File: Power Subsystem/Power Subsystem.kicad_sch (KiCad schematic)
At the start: 38 parts, among them J1 Conn_01x16_Pin, J2 Conn_01x02_Pin, Q1 PMOS, SW1 SW_SPST, U1 MCP73831-2-OT

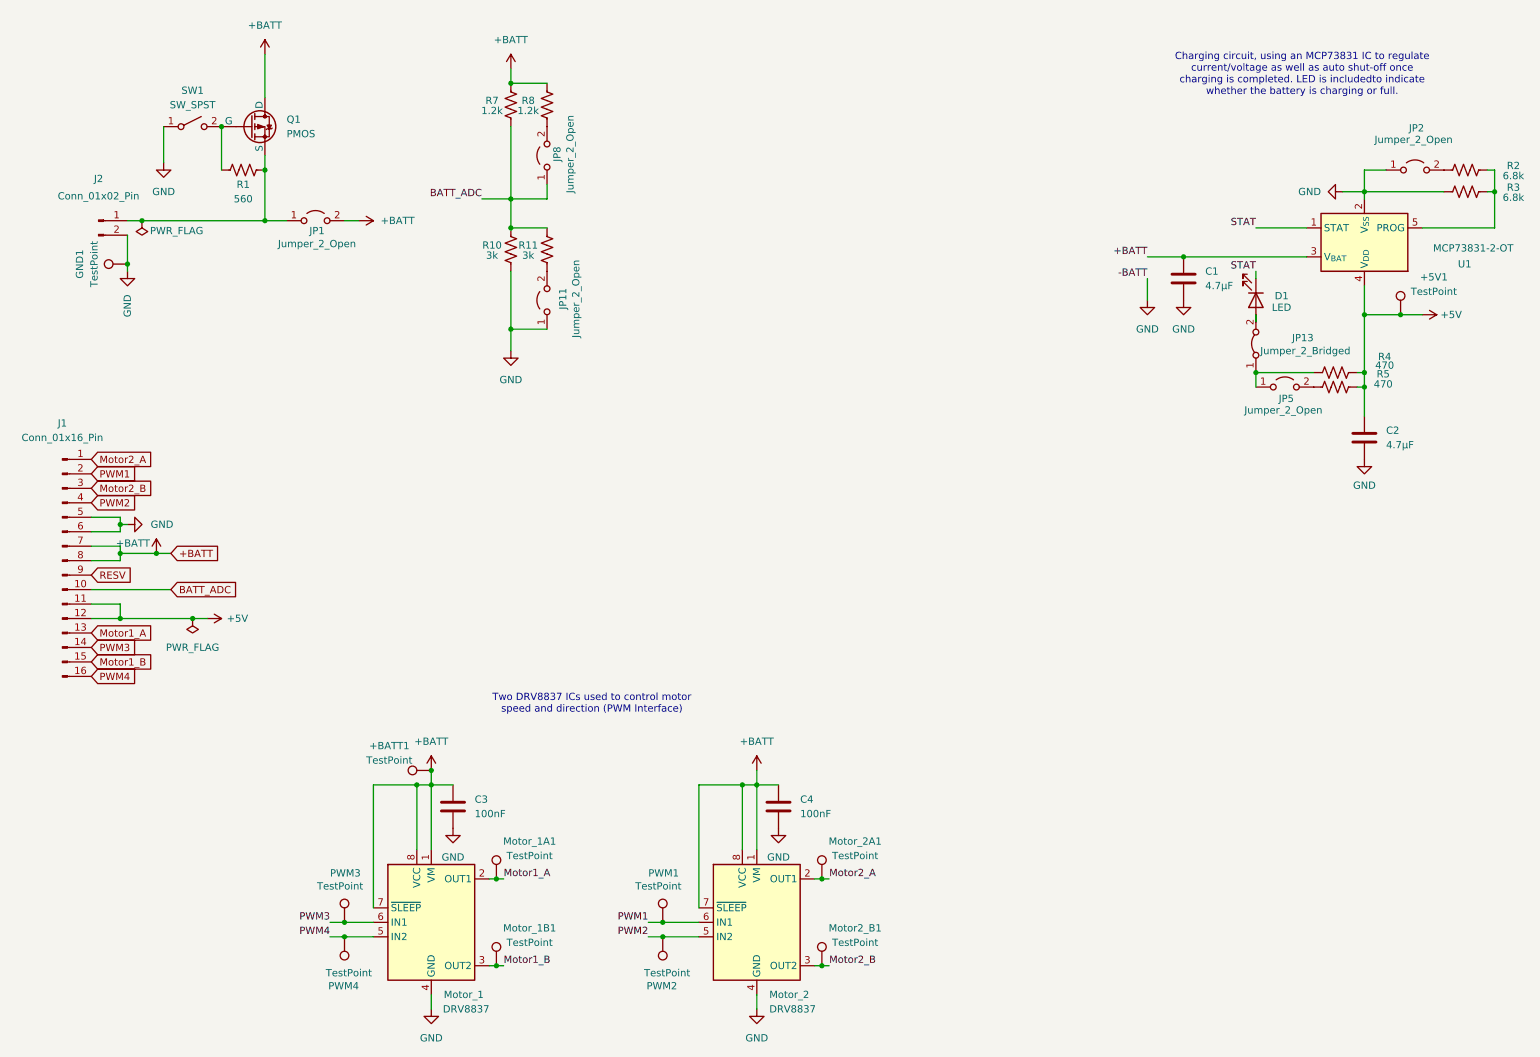
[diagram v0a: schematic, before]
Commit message: Final Schematic and PCB designs
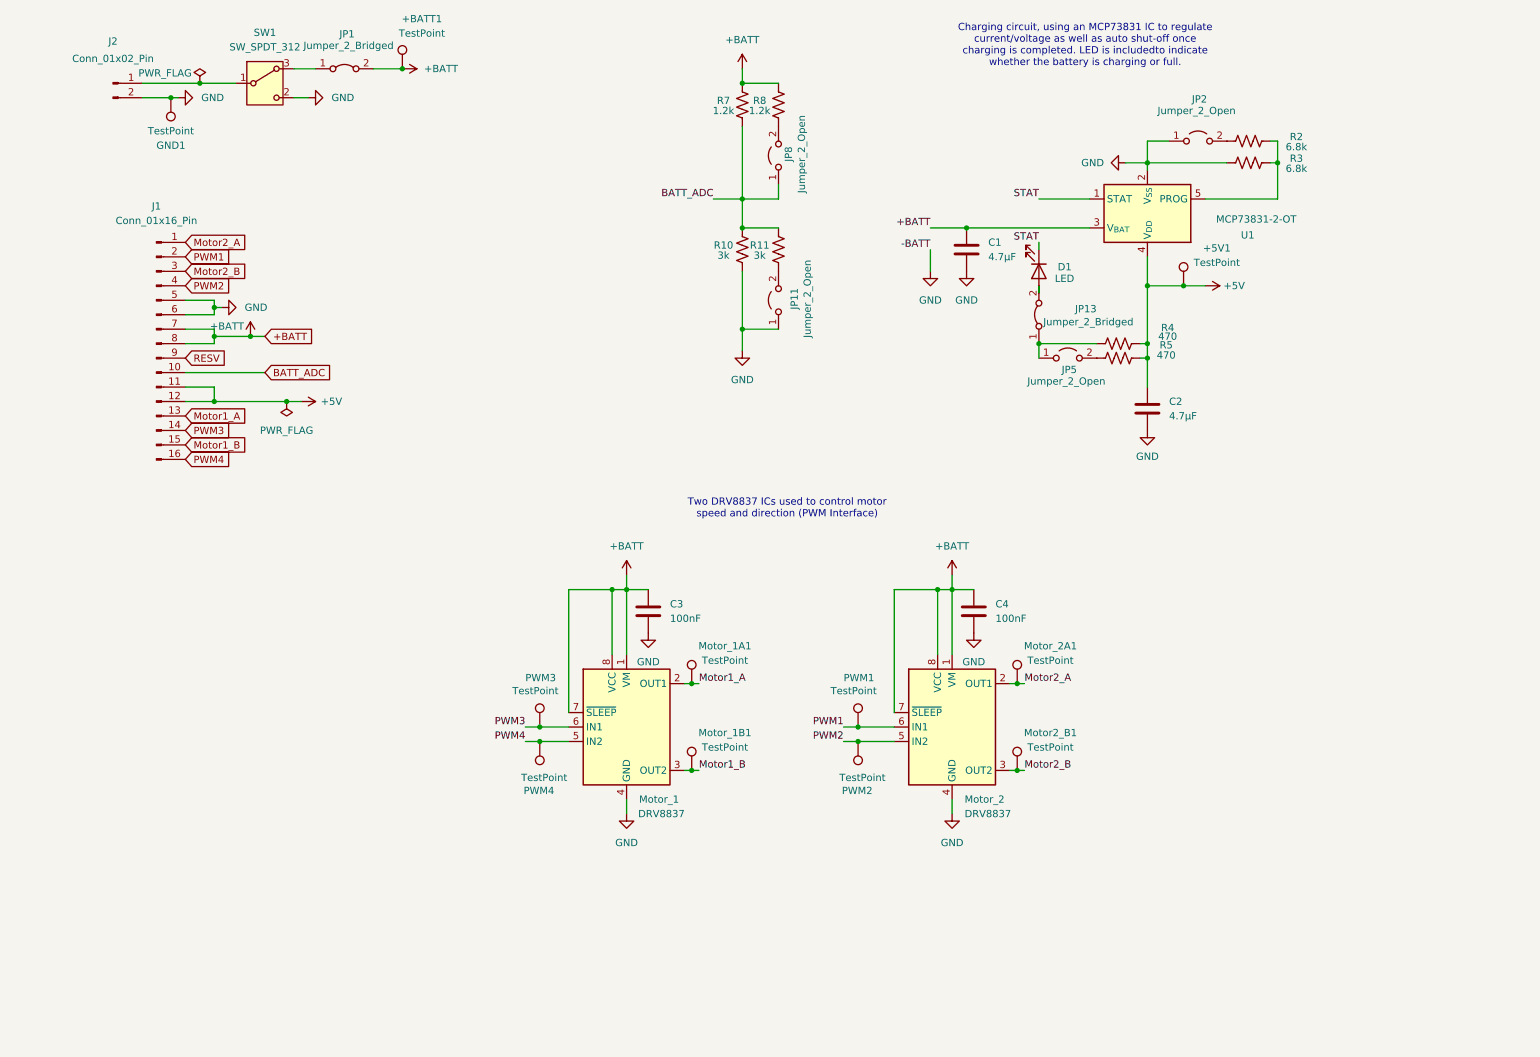
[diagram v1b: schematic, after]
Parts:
- removed JP1: Jumper_2_Open, Jumper:SolderJumper-2_P1.3mm_Open_TrianglePad1.0x1.5mm, symbol Jumper:Jumper_2_Open
- removed Q1: PMOS, Package_TO_SOT_SMD:SOT-23, symbol Simulation_SPICE:PMOS
- removed R1: 560, Resistor_SMD:R_0603_1608Metric, symbol Device:R_US
- removed SW1: SW_SPST, Button_Switch_SMD:SW_DIP_SPSTx01_Slide_Omron_A6S-110x_W8.9mm_P2.54mm, symbol Switch:SW_SPST
- added JP1: Jumper_2_Bridged, Jumper:SolderJumper-2_P1.3mm_Bridged2Bar_RoundedPad1.0x1.5mm, symbol Jumper:Jumper_2_Bridged
- added SW1: SW_SPDT_312, Custom Footprints:SW-TH_SS-12D10L5, symbol Switch:SW_SPDT_312
- D1: footprint LED_THT:LED_D5.0mm -> LED_SMD:LED_0603_1608Metric; LCSC (none) -> C2286
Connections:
- net +BATT: now also JP1.2 (B)
- net GND: now also SW1.2 (C)
- net at J2.1 (Pin_1): now also SW1.1 (B)
- new net: JP1.1 (A), SW1.3 (A)
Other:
- moved on the sheet: +5V1, +BATT1, C1, C2, C3, C4, D1, GND1, J1, J2, JP11, JP13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
